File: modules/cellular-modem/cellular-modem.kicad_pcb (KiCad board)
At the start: 4 copper layers, 42.8 x 71.1 mm, 23 parts, among them J1 MM60-mini-PCIe, J2 MM60-EZH059-B5-R650, U1 TXV0108RGYR, U2 TXV0108RGYR, U3 TXV0108RGYR, U4 TPS631000DRLR, U5 TPS631000DRLR

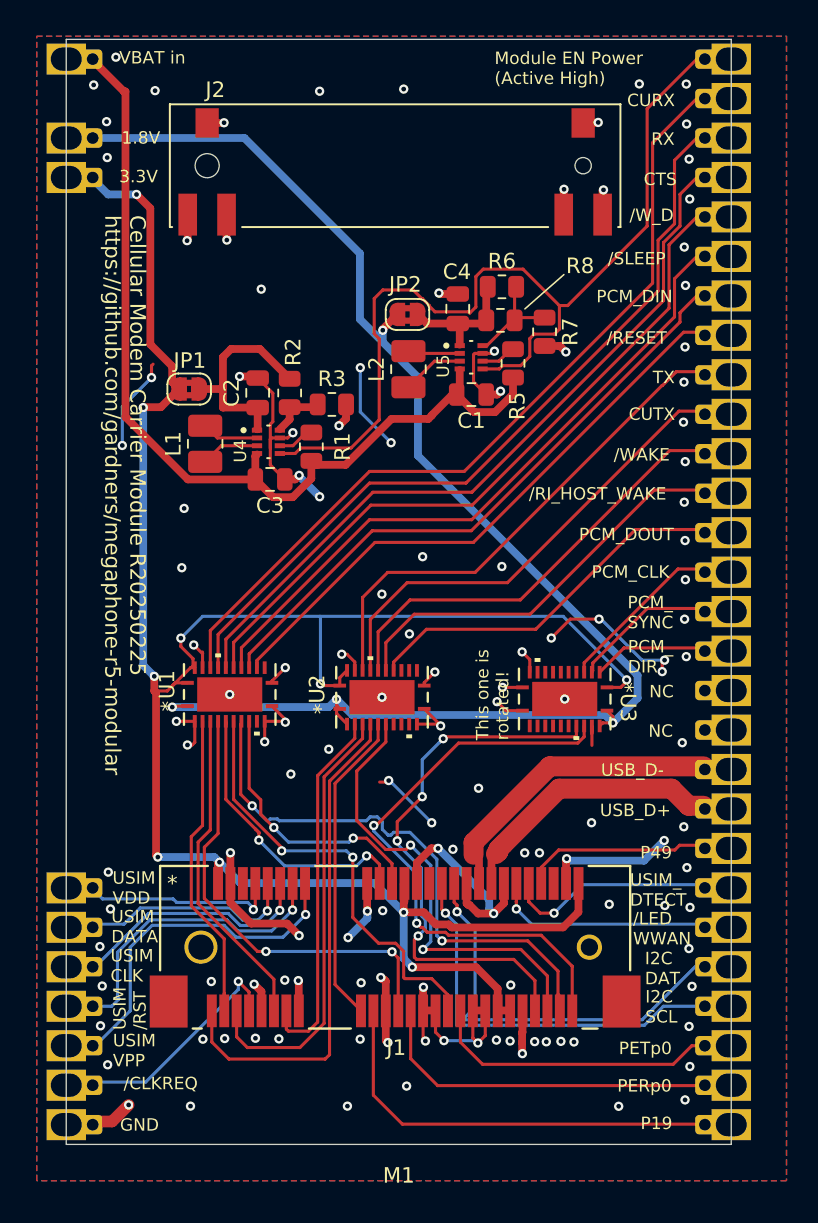
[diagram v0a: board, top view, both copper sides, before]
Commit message: Updating all modules
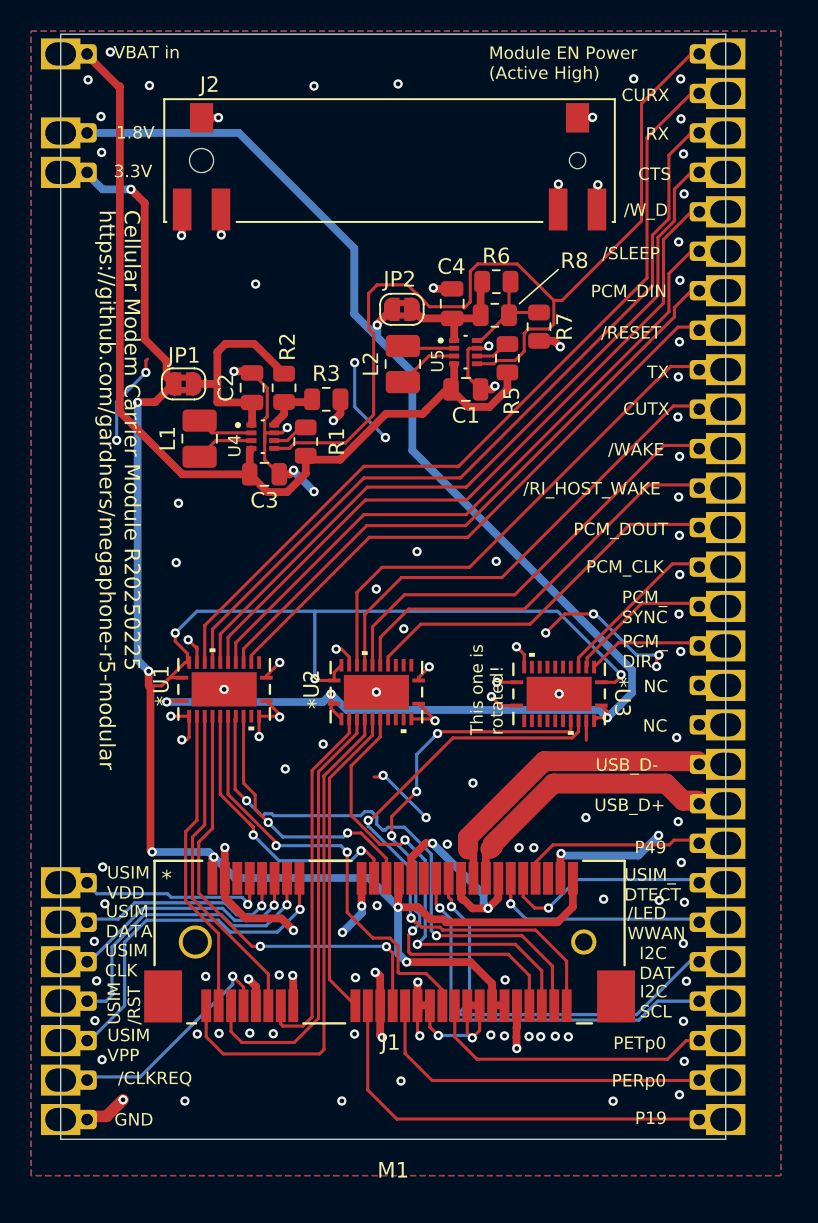
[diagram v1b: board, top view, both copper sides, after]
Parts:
- moved JP2 0.49 mm to (89.5, 53.1)
- moved R2 0.49 mm to (82.0, 58.2)
- moved C1 0.49 mm to (93.7, 58.3)
- moved C2 0.49 mm to (79.9, 58.2)
- moved C3 0.49 mm to (80.7, 63.8)
- moved C4 0.49 mm to (92.8, 52.8)
- moved J1 0.49 mm to (88.8, 93.9)
- moved J2 0.49 mm to (88.8, 43.6)
- moved JP1 0.49 mm to (75.5, 57.9)
- moved L1 0.49 mm to (76.5, 61.5)
- moved L2 0.49 mm to (89.6, 56.7)
- moved M1 0.49 mm to (89.0, 71.0)
- moved R1 0.49 mm to (83.4, 61.6)
- moved R3 0.49 mm to (84.7, 58.9)
- moved R5 0.49 mm to (96.3, 56.3)
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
